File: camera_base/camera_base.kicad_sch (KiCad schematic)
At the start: 19 parts, among them J1 Raspberry_Pi_4, J2 Conn_02x03_Odd_Even, SW1 SW_Push_Dual, SW2 SW_Push_Dual, SW3 SW_Push_Dual, SW5 SW_Push_Dual

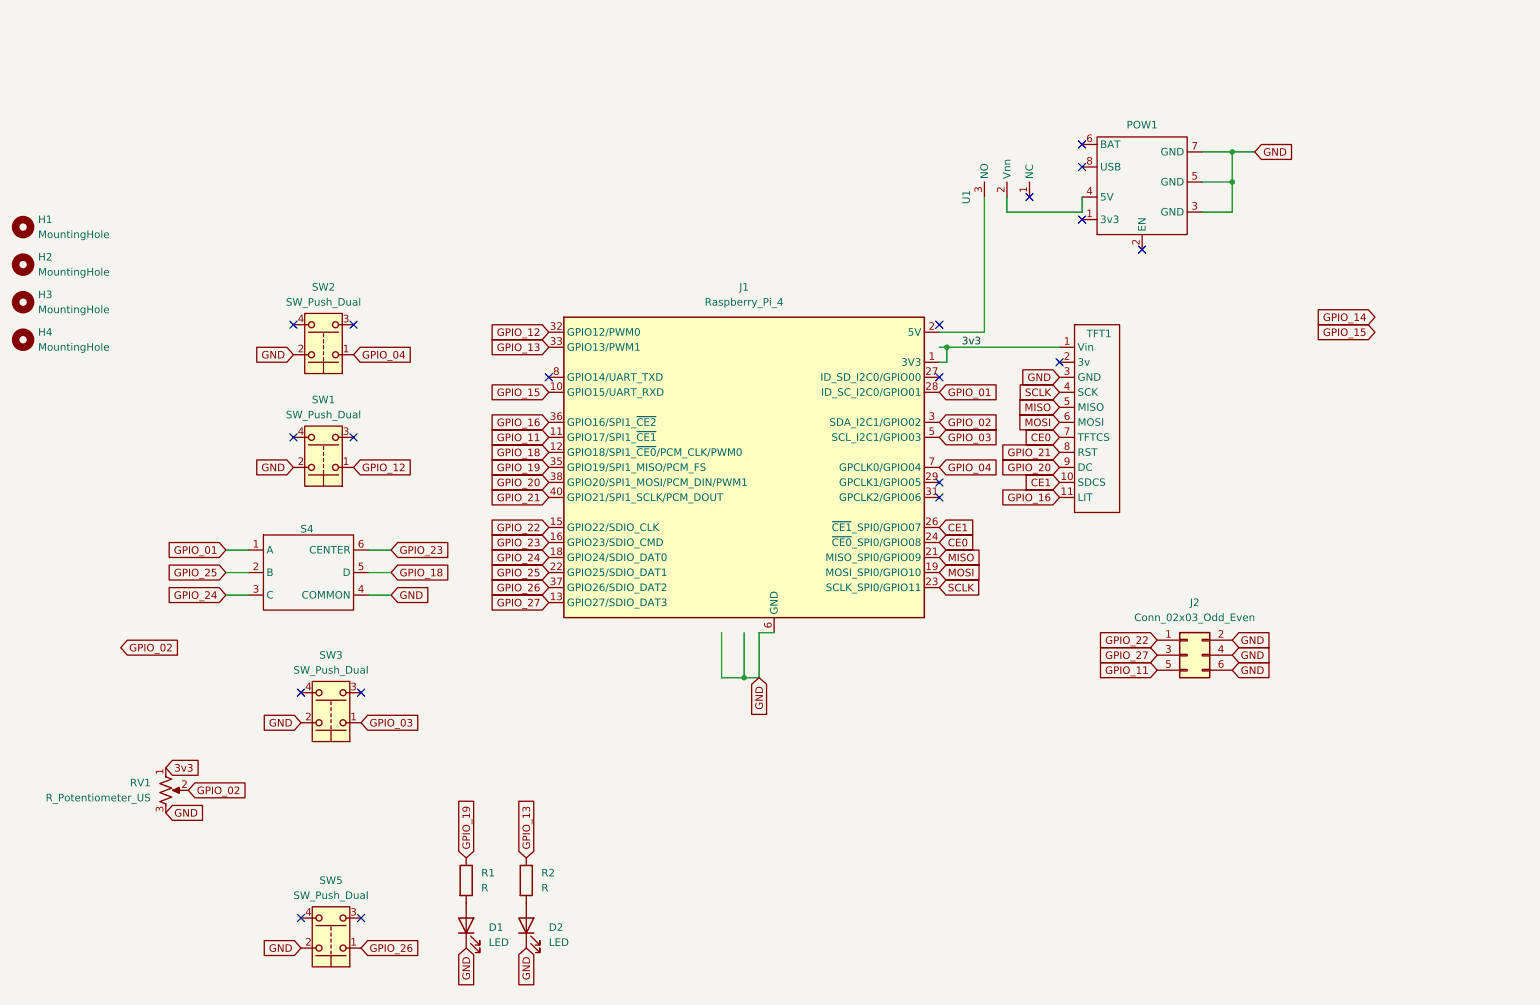
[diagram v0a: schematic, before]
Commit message: update
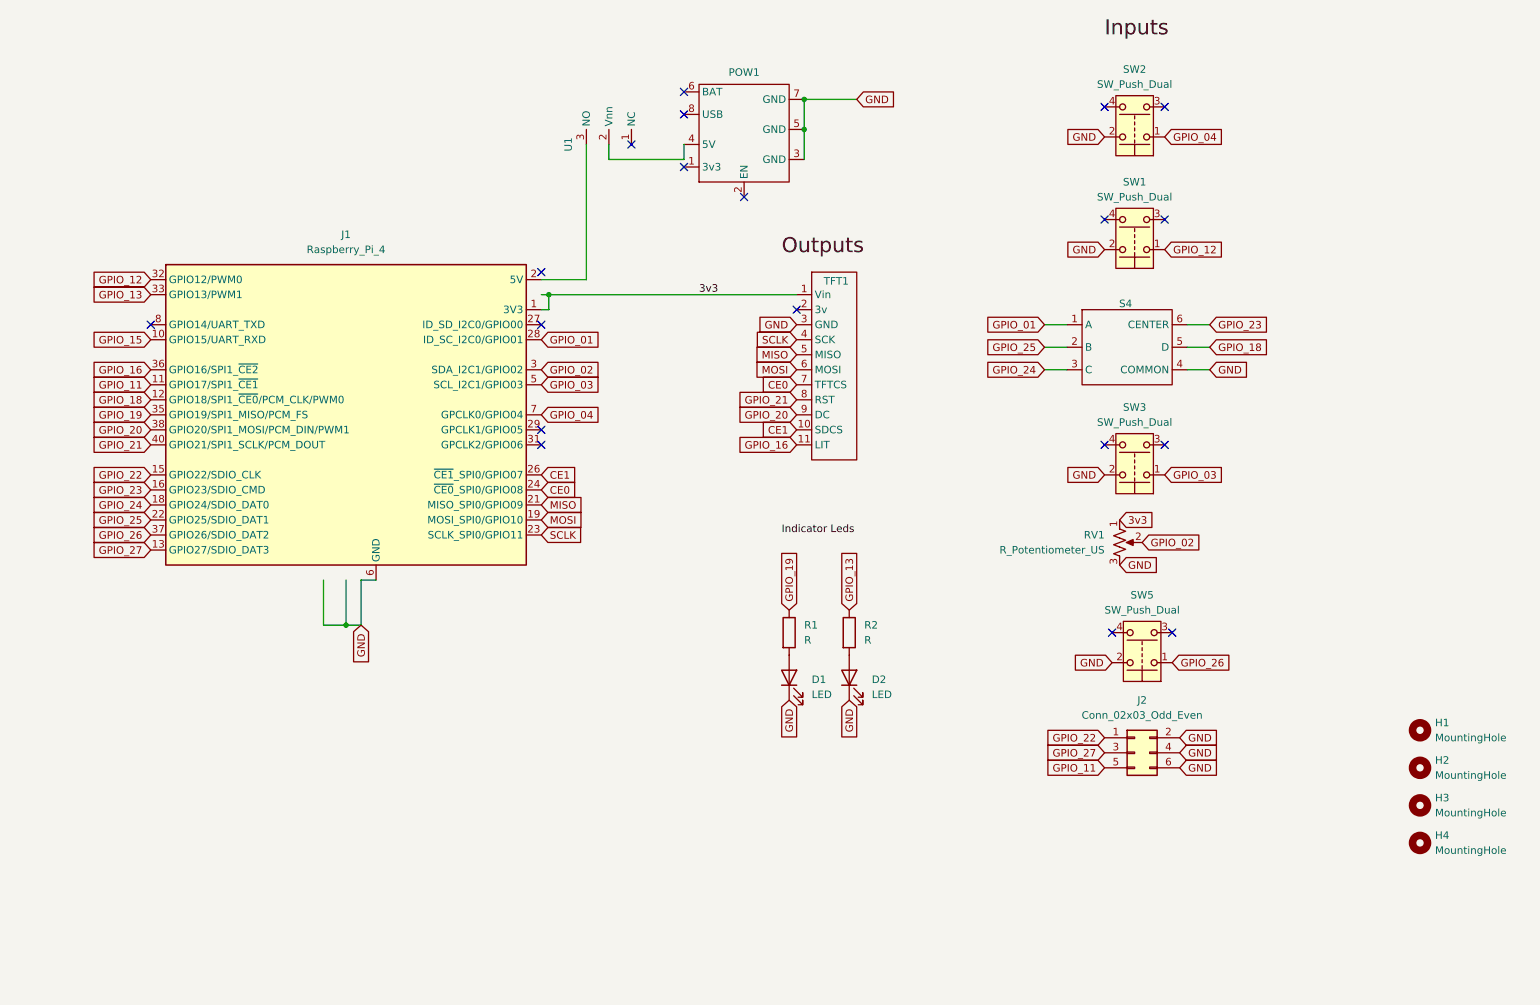
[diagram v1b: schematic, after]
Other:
- moved on the sheet: D1, D2, H1, H2, H3, H4, J1, J2, POW1, R1, R2, RV1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
